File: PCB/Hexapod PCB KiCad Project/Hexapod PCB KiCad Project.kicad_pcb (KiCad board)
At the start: 2 copper layers, 3 parts, among them J1 Male Pin Header 1x3, J2 Power Terminal, U1 DEV-16771

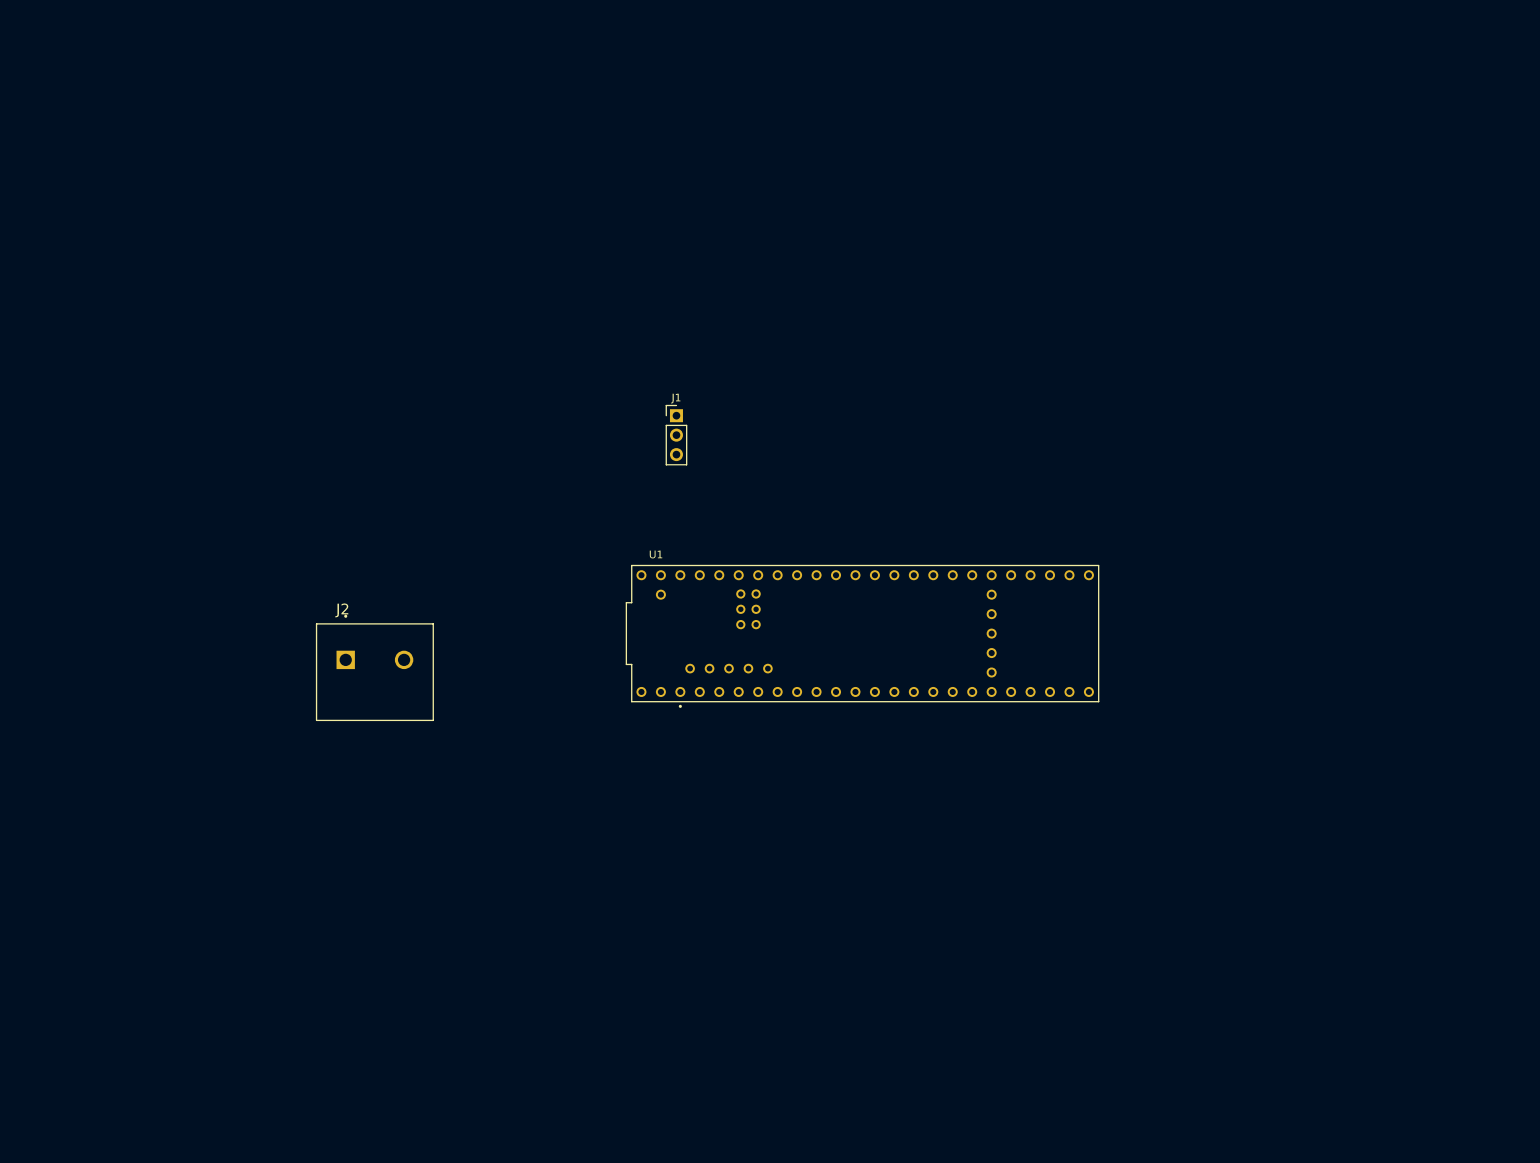
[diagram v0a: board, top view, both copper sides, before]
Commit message: Pcb updates
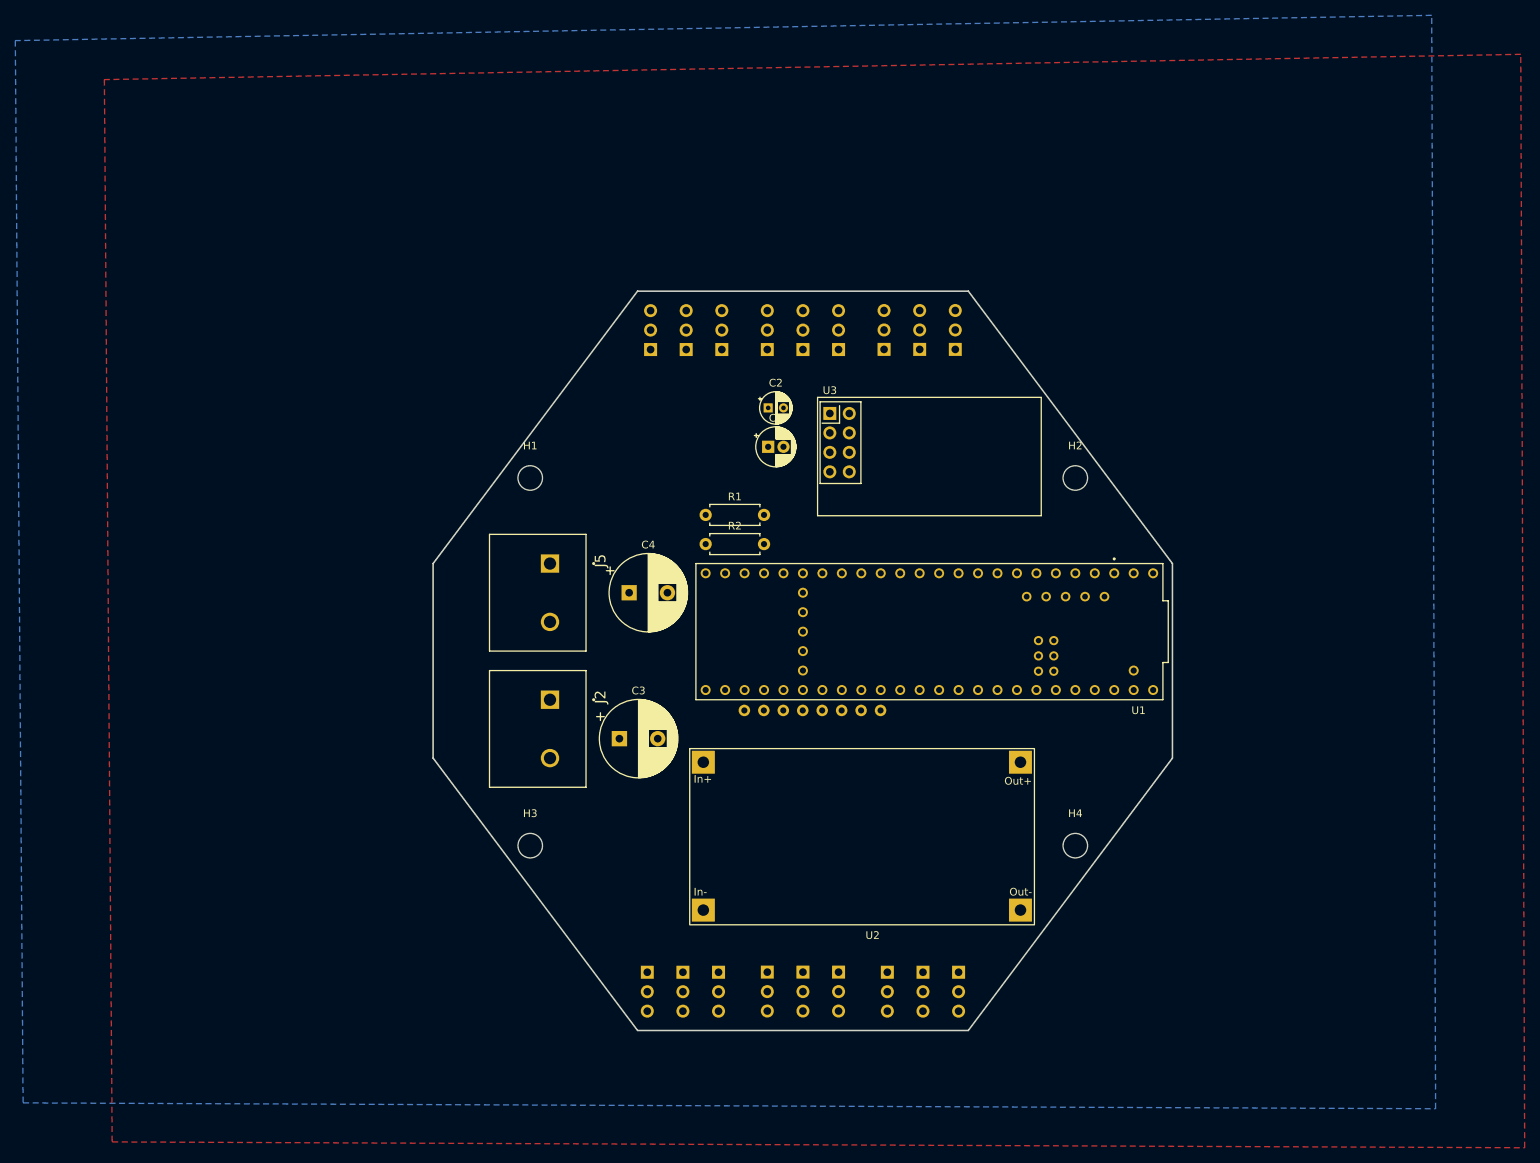
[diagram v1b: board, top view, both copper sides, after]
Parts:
- added C1: 50V 10uF, Capacitor_THT:CP_Radial_D5.0mm_P2.00mm, F.Cu at (139.0, 73.7)
- added C2: 50V 0.1uF, Capacitor_THT:CP_Radial_D4.0mm_P2.00mm, F.Cu at (139.0, 68.6)
- added C3: 16V 1000uf, Capacitor_THT:CP_Radial_D10.0mm_P5.00mm, F.Cu at (119.6, 111.8)
- added C4: 16V 1000uf, Capacitor_THT:CP_Radial_D10.0mm_P5.00mm, F.Cu at (120.8, 92.7)
- added H1: MountingHole, MountingHole:MountingHole_3.2mm_M3, F.Cu at (107.9, 77.7)
- added H2: MountingHole, MountingHole:MountingHole_3.2mm_M3, F.Cu at (179.1, 77.7)
- added H3: MountingHole, MountingHole:MountingHole_3.2mm_M3, F.Cu at (107.9, 125.7)
- added H4: MountingHole, MountingHole:MountingHole_3.2mm_M3, F.Cu at (179.1, 125.7)
- added J10: Conn_01x03, Connector_PinHeader_2.54mm:PinHeader_1x03_P2.54mm_Vertical, B.Cu at (127.8, 142.3)
- added J11: Conn_01x03, Connector_PinHeader_2.54mm:PinHeader_1x03_P2.54mm_Vertical, B.Cu at (123.2, 142.3)
- added J12: Conn_01x03, Connector_PinHeader_2.54mm:PinHeader_1x03_P2.54mm_Vertical, B.Cu at (123.6, 61.0)
- added J13: Conn_01x03, Connector_PinHeader_2.54mm:PinHeader_1x03_P2.54mm_Vertical, B.Cu at (128.3, 61.0)
- added J14: Conn_01x03, Connector_PinHeader_2.54mm:PinHeader_1x03_P2.54mm_Vertical, B.Cu at (132.9, 61.0)
- added J15: Conn_01x03, Connector_PinHeader_2.54mm:PinHeader_1x03_P2.54mm_Vertical, B.Cu at (138.9, 61.0)
- added J16: Conn_01x03, Connector_PinHeader_2.54mm:PinHeader_1x03_P2.54mm_Vertical, B.Cu at (143.5, 61.0)
- added J17: Conn_01x03, Connector_PinHeader_2.54mm:PinHeader_1x03_P2.54mm_Vertical, B.Cu at (148.2, 61.0)
- added J18: Conn_01x03, Connector_PinHeader_2.54mm:PinHeader_1x03_P2.54mm_Vertical, B.Cu at (154.1, 60.9)
- added J19: Conn_01x03, Connector_PinHeader_2.54mm:PinHeader_1x03_P2.54mm_Vertical, B.Cu at (158.8, 60.9)
- added J20: Conn_01x03, Connector_PinHeader_2.54mm:PinHeader_1x03_P2.54mm_Vertical, B.Cu at (163.4, 60.9)
- added J3: Conn_01x03, Connector_PinHeader_2.54mm:PinHeader_1x03_P2.54mm_Vertical, B.Cu at (159.2, 142.3)
- added J4: Conn_01x03, Connector_PinHeader_2.54mm:PinHeader_1x03_P2.54mm_Vertical, B.Cu at (154.5, 142.3)
- added J5: Switch, Terminal 2 Pin:CUI_TB005-762-02BE, F.Cu at (110.5, 88.9)
- added J6: Conn_01x03, Connector_PinHeader_2.54mm:PinHeader_1x03_P2.54mm_Vertical, B.Cu at (148.2, 142.2)
- added J7: Conn_01x03, Connector_PinHeader_2.54mm:PinHeader_1x03_P2.54mm_Vertical, B.Cu at (143.5, 142.2)
- added J8: Conn_01x03, Connector_PinHeader_2.54mm:PinHeader_1x03_P2.54mm_Vertical, B.Cu at (138.9, 142.2)
- added J9: Conn_01x03, Connector_PinHeader_2.54mm:PinHeader_1x03_P2.54mm_Vertical, B.Cu at (132.5, 142.3)
- added R1: 10k, Resistor_THT:R_Axial_DIN0207_L6.3mm_D2.5mm_P7.62mm_Horizontal, F.Cu at (130.8, 82.5)
- added R2: 22k, Resistor_THT:R_Axial_DIN0207_L6.3mm_D2.5mm_P7.62mm_Horizontal, F.Cu at (130.8, 86.4)
- added U2: Voltage Regulator, Voltage Regulator LM2596:Voltage Regulator LM2596, F.Cu at (128.7, 113.1)
- added U3: NRF24L01_Breakout, RF_Module:nRF24L01_Breakout, F.Cu at (147.0, 69.3)
- added U4: Gyro, MPU6050 THT:MPU6050 THT, B.Cu at (132.1, 101.9)
- J1: value Male Pin Header 1x3 -> Conn_01x03; moved to B.Cu
- J2: value Power Terminal -> Battery
- U1: footprint TEENSY 4.1:MODULE_DEV-16771 -> Teensy 4.1:MODULE_DEV-16771
- moved J1 81.5 mm to (163.8, 142.3), turned to 180 degrees
- moved J2 27.2 mm to (110.5, 106.7), turned to -90 degrees
- moved U1 8.39 mm to (160.0, 97.8), turned to 180 degrees
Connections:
- net Net-(U1-3.3V-Pad3.3V_1) renamed +3.3V
- J1 pad 1: unconnected-(J1-Pin_1-Pad1) -> GND
- J1 pad 2: unconnected-(J1-Pin_2-Pad2) -> +BATT
- J1 pad 3: unconnected-(J1-Pin_3-Pad3) -> Leg1 Coxa
- J2 pad 1: unconnected-(J2-Pad1) -> GND
- J2 pad 2: unconnected-(J2-Pad2) -> Net-(J2-Pad2)
- U1 pad 10: unconnected-(U1-CS1-Pad10) -> Leg1 Tibia
- U1 pad 11: unconnected-(U1-MOSI-Pad11) -> MOSI
- U1 pad 12: unconnected-(U1-MISO-Pad12) -> MISO
- U1 pad 13: unconnected-(U1-SCK-Pad13) -> SCK
- U1 pad 14: unconnected-(U1-A0-Pad14) -> Leg6 Femur
- U1 pad 15: unconnected-(U1-A1-Pad15) -> Leg6 Coxa
- U1 pad 16: unconnected-(U1-A2-Pad16) -> Battery Voltage Divider
- U1 pad 18: unconnected-(U1-A4-Pad18) -> Gyro SDA
- U1 pad 19: unconnected-(U1-A5-Pad19) -> Gyro SCL
- U1 pad 2: unconnected-(U1-OUT2-Pad2) -> Leg3 Coxa
- U1 pad 24: unconnected-(U1-A10-Pad24) -> Leg4 Tibia
- U1 pad 25: unconnected-(U1-A11-Pad25) -> Leg4 Femur
- U1 pad 26: unconnected-(U1-A12-Pad26) -> CE
- U1 pad 27: unconnected-(U1-A13-Pad27) -> CSN
- U1 pad 28: unconnected-(U1-RX7-Pad28) -> Leg4 Coxa
- U1 pad 29: unconnected-(U1-TX7-Pad29) -> Leg5 Tibia
- U1 pad 3: unconnected-(U1-LRCLK2-Pad3) -> Leg3 Femur
- U1 pad 33: unconnected-(U1-MCLK2-Pad33) -> Leg5 Femur
- U1 pad 36: unconnected-(U1-CS2-Pad36) -> Leg5 Coxa
- U1 pad 37: unconnected-(U1-CS3-Pad37) -> Leg6 Tibia
- U1 pad 4: unconnected-(U1-BCLK2-Pad4) -> Leg3 Tibia
- U1 pad 5: unconnected-(U1-IN2-Pad5) -> Leg2 Coxa
- U1 pad 5V: unconnected-(U1-Pad5V) -> +5V
- U1 pad 6: unconnected-(U1-OUT1D-Pad6) -> Leg2 Femur
- U1 pad 7: unconnected-(U1-RX2-Pad7) -> Leg2 Tibia
- U1 pad 8: unconnected-(U1-TX2-Pad8) -> Leg1 Coxa
- U1 pad 9: unconnected-(U1-OUT1C-Pad9) -> Leg1 Femur
- U1 pad GND1: Net-(U1-GND-PadGND1) -> GND
- U1 pad GND2: Net-(U1-GND-PadGND1) -> GND
- U1 pad GND3: Net-(U1-GND-PadGND1) -> GND
- U1 pad GND4: Net-(U1-GND-PadGND1) -> GND
- U1 pad GND5: Net-(U1-GND-PadGND1) -> GND
- U1 pad VIN: unconnected-(U1-PadVIN) -> Teensy VIN
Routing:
- added copper zone on F.Cu, net (none)
- added copper zone on B.Cu, net GND
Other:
- board outline added: 96.5 x 96.5 mm
